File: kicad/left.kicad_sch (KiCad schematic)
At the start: 102 parts, among them Q1 PMF170XP,115, Q2 FS8205A_C2830320, SW1 TS-1088-AR02016, U1 SN74LVC1G17DBVR, U2 E73-2G4M08S1C, U3 SN74LVC1G74DQER, U4 S2B-PH-K-S(LF)(SN), U5 BL8573CS8TR, U6 DW01A_C42380662, U7 LP5024RSMR, U8 MAX17048, U9 USBLC6-2SC6, X1 FC-13532.768KHZ9PF20PPM

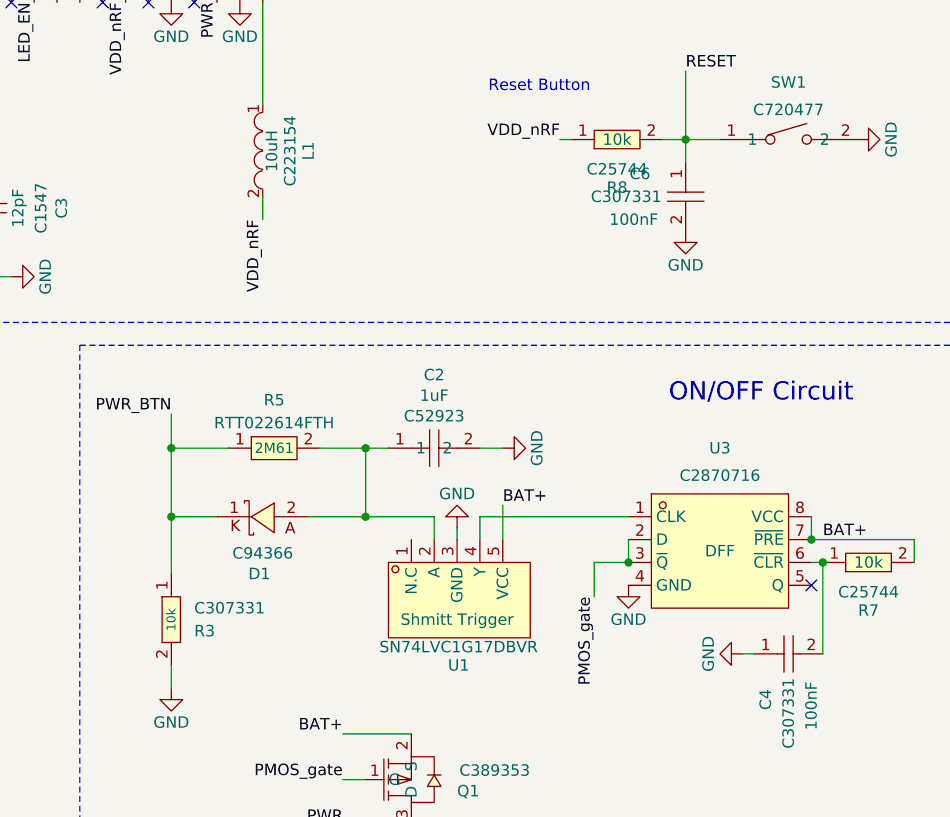
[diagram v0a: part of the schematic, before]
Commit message: ... todo: update panel woth newest left and right pcb
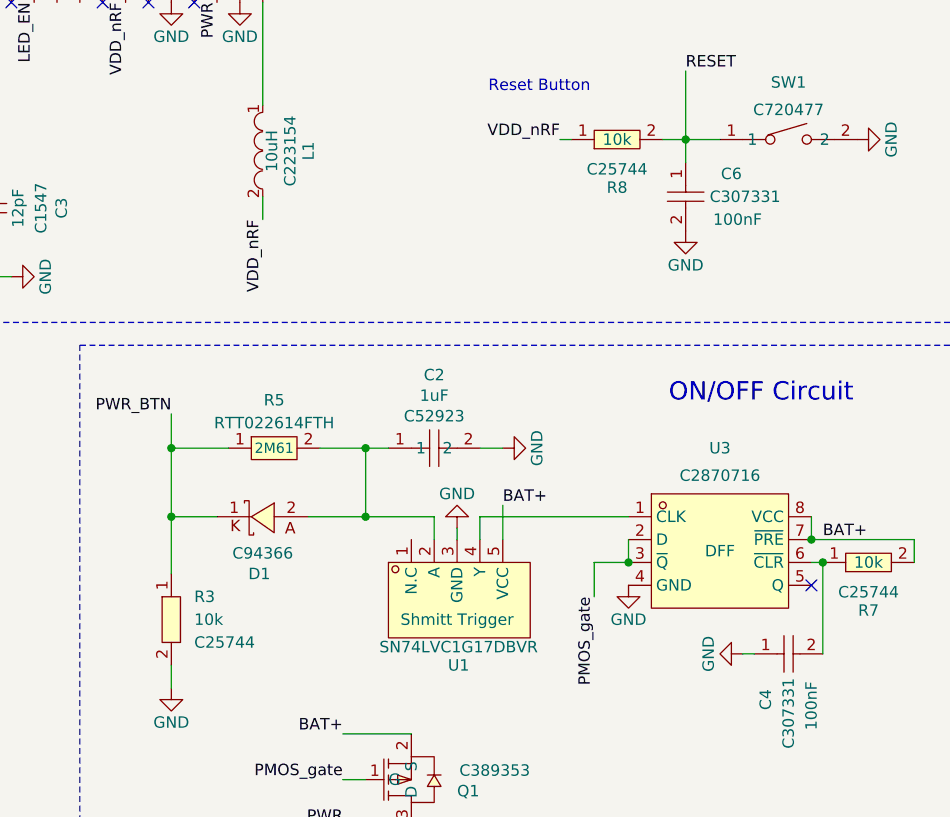
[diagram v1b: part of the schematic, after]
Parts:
- removed R3: 0402WGF1002TCE, easyeda2kicad:R0402, symbol easyeda2kicad:RC0402FR-07100KL
- added R3: 0402WGF1002TCE, easyeda2kicad:R0402, symbol easyeda2kicad:RC0402FR-0710KL
- S1, S10, S11, S12, S13, S14, S15, S16, S17, S18, S19, S2, S20, S3, S4, S5, S6, S7, S8, S9: footprint hexcaps:PG1350_hotswap -> hexcaps:PG1350_hotswap_reversed
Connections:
- net GND: now also R3.2
- net PWR_BTN: now also R3.1
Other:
- moved on the sheet: C6
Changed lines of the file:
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@@
 			)
 		)
-		(property "Footprint" "hexcaps:PG1350_hotswap"
+		(property "Footprint" "hexcaps:PG1350_hotswap_reversed"
 			(at 74.422 282.448 0)
 			(hide yes)
@@
 			)
 		)
-		(property "Footprint" "hexcaps:PG1350_hotswap"
+		(property "Footprint" "hexcaps:PG1350_hotswap_reversed"
 			(at 74.422 206.248 0)
 			(hide yes)
@@
 			)
 		)
-		(property "Footprint" "hexcaps:PG1350_hotswap"
+		(property "Footprint" "hexcaps:PG1350_hotswap_reversed"
 			(at 74.422 257.048 0)
 			(hide yes)
@@
 			)
 		)
-		(property "Footprint" "hexcaps:PG1350_hotswap"
+		(property "Footprint" "hexcaps:PG1350_hotswap_reversed"
 			(at 36.322 257.048 0)
 			(hide yes)
@@
 	)
 	(symbol
-		(lib_id "easyeda2kicad:RC0402FR-07100KL")
-		(at 316.23 139.7 90)
-		(mirror x)
-		(unit 1)
-		(body_style 1)
-		(exclude_from_sim no)
-		(in_bom yes)
-		(on_board yes)
-		(in_pos_files yes)
-		(dnp no)
-		(fields_autoplaced yes)
-		(property "Reference" "R3"
-			(at 318.77 140.9701 90)
-			(show_name no)
-			(do_not_autoplace no)
-			(effects
-				(font
-					(size 1.27 1.27)
-				)
-				(justify right)
-			)
-		)
-		(property "Value" "0402WGF1002TCE"
-			(at 312.42 139.7 0)
-			(hide yes)
-			(show_name no)
-			(do_not_autoplace no)
-			(effects
-				(font
-					(size 1.27 1.27)
-				)
-			)
-		)
-		(property "Footprint" "easyeda2kicad:R0402"
-			(at 323.85 139.7 0)
-			(hide yes)
-			(show_name no)
-			(do_not_autoplace no)
-			(effects
-				(font
-					(size 1.27 1.27)
-				)
-			)
-		)
-		(property "Datasheet" "https://lcsc.com/datasheet/C25744.pdf"
-			(at 326.39 139.7 0)
-			(hide yes)
-			(show_name no)
-			(do_not_autoplace no)
-			(effects
-				(font
-					(size 1.27 1.27)
-				)
-			)
-		)
-		(property "Description" "10k"
-			(at 316.23 139.7 0)
-			(show_name no)
-			(do_not_autoplace no)
-			(effects
-				(font
-					(size 1 1)
-				)
-			)
-		)
-		(property "LCSC Part" "C307331"
-			(at 318.77 138.4301 90)
-			(show_name no)
-			(do_not_autoplace no)
-			(effects
-				(font
-					(size 1.27 1.27)
-				)
-				(justify right)
-			)
-		)
-		(pin "1"
-		)
-		(pin "2"
-		)
-		(instances
-			(project "left"
-				(path "/3171f1b4-f2dd-4471-8b63-415e18370dba"
-					(reference "R3")
-					(unit 1)
-				)
-			)
-		)
-	)
-	(symbol
 		(lib_name "LPT67F-P1R2-35-Z_14")
 		(lib_id "easyeda2kicad:LPT67F-P1R2-35-Z")
@@
 		(lib_name "GRM033C71C104KE14D_19")
 		(lib_id "easyeda2kicad:GRM033C71C104KE14D")
-		(at 373.38 92.71 90)
-		(mirror x)
+		(at 373.38 92.71 270)
 		(unit 1)
 		(body_style 1)
@@
 		(dnp no)
 		(property "Reference" "C6"
-			(at 368.3 90.17 90)
+			(at 378.46 90.17 90)
 			(show_name no)
 			(do_not_autoplace no)
@@
 		)
 		(property "Value" "CL05B104KB54PNC"
-			(at 369.57 92.71 0)
+			(at 377.19 92.71 0)
 			(hide yes)
 			(show_name no)
@@
 		)
 		(property "Footprint" "easyeda2kicad:C0402"
-			(at 381 92.71 0)
+			(at 365.76 92.71 0)
 			(hide yes)
 			(show_name no)
@@
 		)
 		(property "Datasheet" "https://lcsc.com/datasheet/C307331.pdf"
-			(at 383.54 92.71 0)
+			(at 363.22 92.71 0)
 			(hide yes)
 			(show_name no)
@@
 		)
 		(property "Description" "100nF"
-			(at 370.332 95.25 90)
+			(at 376.428 95.25 90)
 			(show_name no)
 			(do_not_autoplace no)
@@
 		)
 		(property "LCSC Part" "C307331"
-			(at 366.776 92.71 90)
+			(at 379.984 92.71 90)
 			(show_name no)
 			(do_not_autoplace no)
@@
 			)
 		)
-		(property "Footprint" "hexcaps:PG1350_hotswap"
+		(property "Footprint" "hexcaps:PG1350_hotswap_reversed"
 			(at 112.522 257.048 0)
 			(hide yes)
@@
 			)
 		)
-		(property "Footprint" "hexcaps:PG1350_hotswap"
+		(property "Footprint" "hexcaps:PG1350_hotswap_reversed"
 			(at 229.362 204.978 0)
 			(hide yes)
@@
 			)
 		)
-		(property "Footprint" "hexcaps:PG1350_hotswap"
+		(property "Footprint" "hexcaps:PG1350_hotswap_reversed"
 			(at 36.322 206.248 0)
 			(hide yes)
@@
 			)
 		)
-		(property "Footprint" "hexcaps:PG1350_hotswap"
+		(property "Footprint" "hexcaps:PG1350_hotswap_reversed"
 			(at 150.622 206.248 0)
 			(hide yes)
@@
 			)
 		)
-		(property "Footprint" "hexcaps:PG1350_hotswap"
+		(property "Footprint" "hexcaps:PG1350_hotswap_reversed"
 			(at 188.722 206.248 0)
 			(hide yes)
@@
 			)
 		)
-		(property "Footprint" "hexcaps:PG1350_hotswap"
+		(property "Footprint" "hexcaps:PG1350_hotswap_reversed"
 			(at 150.622 257.048 0)
 			(hide yes)
@@
 			)
 		)
-		(property "Footprint" "hexcaps:PG1350_hotswap"
+		(property "Footprint" "hexcaps:PG1350_hotswap_reversed"
 			(at 188.722 257.048 0)
 			(hide yes)
@@
 			)
 		)
-		(property "Footprint" "hexcaps:PG1350_hotswap"
+		(property "Footprint" "hexcaps:PG1350_hotswap_reversed"
 			(at 112.522 282.448 0)
 			(hide yes)
@@
 	)
 	(symbol
+		(lib_name "RC0402FR-0710KL_1")
+		(lib_id "easyeda2kicad:RC0402FR-0710KL")
+		(at 316.23 139.7 90)
+		(mirror x)
+		(unit 1)
+		(body_style 1)
+		(exclude_from_sim no)
+		(in_bom yes)
+		(on_board yes)
+		(in_pos_files yes)
+		(dnp no)
+		(fields_autoplaced yes)
+		(property "Reference" "R3"
+			(at 318.77 137.1599 90)
+			(show_name no)
+			(do_not_autoplace no)
+			(effects
+				(font
+					(size 1.27 1.27)
+				)
+				(justify right)
+			)
+		)
+		(property "Value" "0402WGF1002TCE"
+			(at 312.42 139.7 0)
+			(hide yes)
+			(show_name no)
+			(do_not_autoplace no)
+			(effects
+				(font
+					(size 1.27 1.27)
+				)
+			)
+		)
+		(property "Footprint" "easyeda2kicad:R0402"
+			(at 323.85 139.7 0)
+			(hide yes)
+			(show_name no)
+			(do_not_autoplace no)
+			(effects
+				(font
+					(size 1.27 1.27)
+				)
+			)
+		)
+		(property "Datasheet" "https://lcsc.com/datasheet/C25744.pdf"
+			(at 326.39 139.7 0)
+			(hide yes)
+			(show_name no)
+			(do_not_autoplace no)
+			(effects
+				(font
+					(size 1.27 1.27)
+				)
+			)
+		)
+		(property "Description" "10k"
+			(at 318.77 139.6999 90)
+			(show_name no)
+			(do_not_autoplace no)
+			(effects
+				(font
+					(size 1.27 1.27)
+				)
+				(justify right)
+			)
+		)
+		(property "LCSC Part" "C25744"
+			(at 318.77 142.2399 90)
+			(show_name no)
+			(do_not_autoplace no)
+			(effects
+				(font
+					(size 1.27 1.27)
+				)
+				(justify right)
+			)
+		)
+		(pin "1"
+		)
+		(pin "2"
+		)
+		(instances
+			(project "left"
+				(path "/3171f1b4-f2dd-4471-8b63-415e18370dba"
+					(reference "R3")
+					(unit 1)
+				)
+			)
+		)
+	)
+	(symbol
 		(lib_name "GRM033C71C104KE14D_19")
 		(lib_id "easyeda2kicad:GRM033C71C104KE14D")
@@
 			)
 		)
-		(property "Footprint" "hexcaps:PG1350_hotswap"
+		(property "Footprint" "hexcaps:PG1350_hotswap_reversed"
 			(at 112.522 206.248 0)
 			(hide yes)
@@
 			)
 		)
-		(property "Footprint" "hexcaps:PG1350_hotswap"
+		(property "Footprint" "hexcaps:PG1350_hotswap_reversed"
 			(at 188.722 282.448 0)
 			(hide yes)
@@
 			)
 		)
-		(property "Footprint" "hexcaps:PG1350_hotswap"
+		(property "Footprint" "hexcaps:PG1350_hotswap_reversed"
 			(at 36.322 231.648 0)
 			(hide yes)
@@
 			)
 		)
-		(property "Footprint" "hexcaps:PG1350_hotswap"
+		(property "Footprint" "hexcaps:PG1350_hotswap_reversed"
 			(at 112.522 231.648 0)
 			(hide yes)
@@
 			)
 		)
-		(property "Footprint" "hexcaps:PG1350_hotswap"
+		(property "Footprint" "hexcaps:PG1350_hotswap_reversed"
 			(at 74.422 231.648 0)
 			(hide yes)
@@
 			)
 		)
-		(property "Footprint" "hexcaps:PG1350_hotswap"
+		(property "Footprint" "hexcaps:PG1350_hotswap_reversed"
 			(at 188.722 231.648 0)
 			(hide yes)
@@
 			)
 		)
-		(property "Footprint" "hexcaps:PG1350_hotswap"
+		(property "Footprint" "hexcaps:PG1350_hotswap_reversed"
 			(at 150.622 282.448 0)
 			(hide yes)
@@
 			)
 		)
-		(property "Footprint" "hexcaps:PG1350_hotswap"
+		(property "Footprint" "hexcaps:PG1350_hotswap_reversed"
 			(at 150.622 231.648 0)
 			(hide yes)
